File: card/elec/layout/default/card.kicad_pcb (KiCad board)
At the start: 2 copper layers, 99 x 55 mm, 3 parts

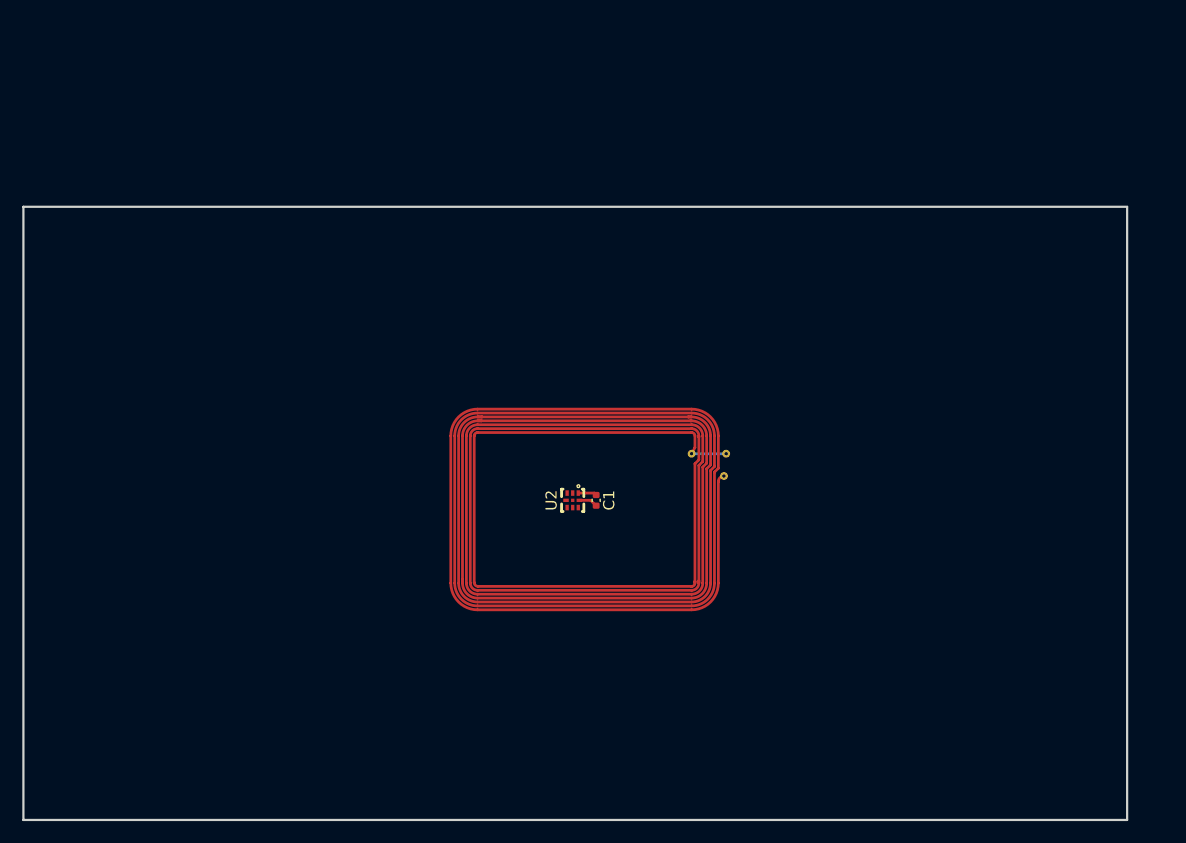
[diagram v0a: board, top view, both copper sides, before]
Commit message: [KICAD] add logo to front
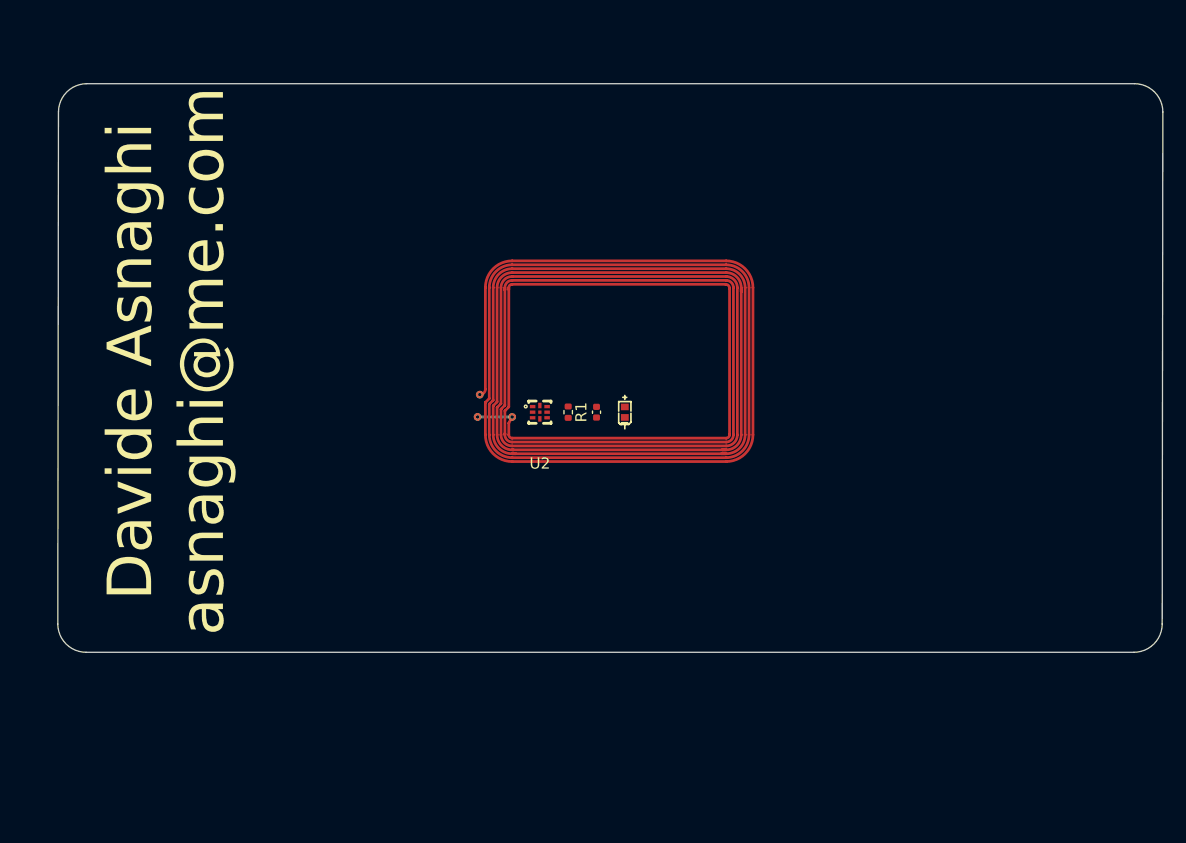
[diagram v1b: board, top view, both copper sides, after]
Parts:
- added LED1: , lib:LED-SMD_L1.0-W0.5-RD, F.Cu at (160.0, 98.0)
- added R1: 62.5mW Thick Film Resistors 50V ±100ppm/℃ ±5% 50Ω 0402 Chip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, lib:R0402, F.Cu at (154.9, 98.0)
- C1: value 50V 50pF C0G ±5% 0402 Multilayer Ceramic Capacitors MLCC - SMD/SMT ROHS -> 16V 220nF X7R ±10% 0402 Multilayer Ceramic Capacitors MLCC - SMD/SMT ROHS
- moved U1 13.7 mm to (159.5, 93.5), turned to 180 degrees
- moved U2 8.44 mm to (152.4, 98.0), turned to 180 degrees
- moved C1 7.91 mm to (157.5, 98.0)
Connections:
- C1 pad 1: la -> vcc
- C1 pad 2: lb -> gnd
- U2 pad 7: vout -> vcc
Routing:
- net lb: track 1.70 -> 0.00 mm
- net la: track 1.68 -> 0.00 mm
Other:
- board size 99 x 55 mm -> 99.1 x 51 mm
- board text added: "Davide Asnaghi asnaghi@me.com"
